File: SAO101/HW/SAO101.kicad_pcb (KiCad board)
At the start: 2 copper layers, 48 x 48 mm, 46 parts, among them J1 USB_B_Micro, J2 SAO_Conn, U1 AMS1117-3.3, U2 MCP23017_SS

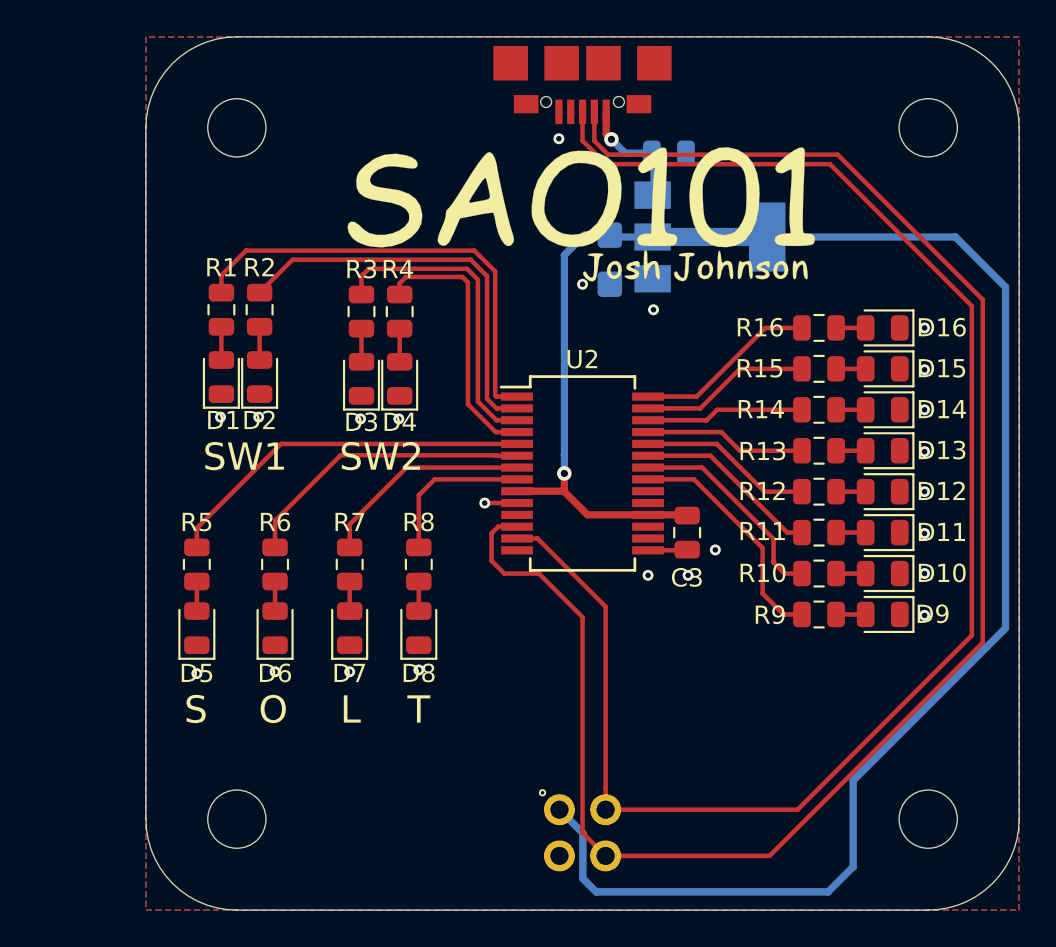
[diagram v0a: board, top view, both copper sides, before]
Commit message: add csides talk
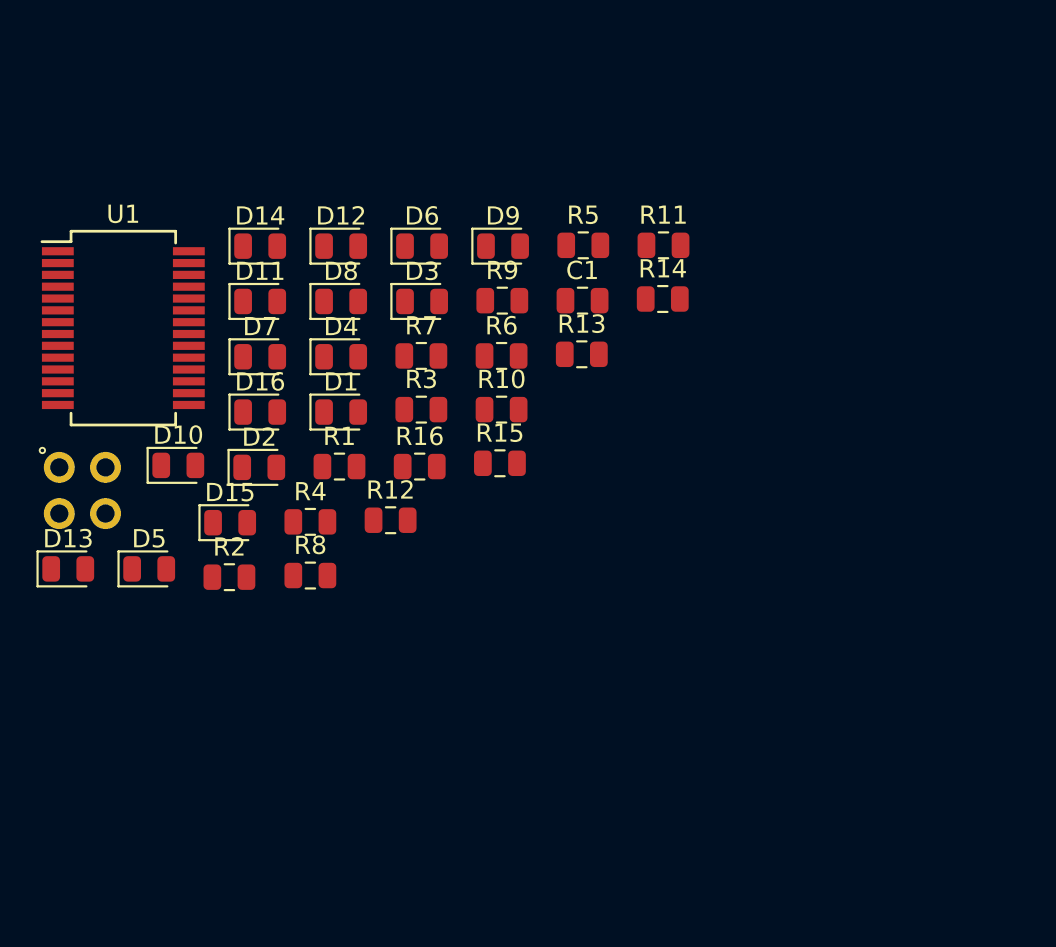
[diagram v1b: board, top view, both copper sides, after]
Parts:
- removed C2: 22u, Capacitor_Tantalum_SMD:CP_EIA-3216-18_Kemet-A
- removed C3: 100n, Capacitor_SMD:C_0805_2012Metric
- removed G***: LOGO, SAO101:josh_img
- removed G***: LOGO, SAO101:SAO101_img
- removed H1, H2, H3, H4: M3, MountingHole:MountingHole_3.2mm_M3_ISO14580
- removed J2: SAO_Conn, SAO101:SAO
- removed REF**: Josh Details, VNA_Footprints:JoshDetails
- removed U2: MCP23017_SS, Package_SO:SSOP-28_5.3x10.2mm_P0.65mm
- C1: value 10u -> 100n; moved to F.Cu
- J1: value USB_B_Micro -> SAO_Conn; footprint VNA_Footprints:MicroUSB_Aliexpress -> SAO101:SAO
- U1: value AMS1117-3.3 -> MCP23017_SS; footprint Package_TO_SOT_SMD:SOT-223-3_TabPin2 -> Package_SO:SSOP-28_5.3x10.2mm_P0.65mm; moved to F.Cu
- moved D13 45.2 mm to (98.7, 89.2), turned to 0 degrees
- moved D10 39.2 mm to (104.8, 83.6), turned to 0 degrees
- moved J1 37.1 mm to (99.5, 84.9), turned to 0 degrees
- moved D15 36.9 mm to (107.6, 86.7), turned to 0 degrees
- moved D11 36.5 mm to (109.3, 74.5), turned to 0 degrees
- moved D14 35.4 mm to (109.3, 71.5), turned to 0 degrees
- moved D16 34.5 mm to (109.3, 80.6), turned to 0 degrees
- moved D12 32.7 mm to (113.7, 71.5), turned to 0 degrees
- moved U1 32.6 mm to (101.8, 76.0)
- moved D9 29.1 mm to (122.6, 71.5), turned to 0 degrees
- moved R5 27.5 mm to (127.0, 71.5), turned to 0 degrees
- moved R9 24.5 mm to (122.6, 74.5), turned to 0 degrees
- moved R12 23.6 mm to (116.5, 86.6), turned to 0 degrees
- moved R16 23.2 mm to (118.0, 83.6), turned to 0 degrees
- moved D6 22.5 mm to (118.2, 71.5), turned to 0 degrees
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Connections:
- C1 pad 1: VBUS -> +3V3
- J1 pad 1: VBUS -> +3V3
- J1 pad 2: /SCL -> GND
- J1 pad 3: /SDA -> /SCL
- J1 pad 4: (no net) -> /SDA
- U1 pad 1: GND -> Net-(R1-Pad2)
- U1 pad 2: +3V3 -> Net-(R2-Pad2)
- U1 pad 3: VBUS -> Net-(R3-Pad2)
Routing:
- net +3V3: track 104.2 -> 0.00 mm, vias 1 -> 0
- net /SCL: track 94.0 -> 0.00 mm
- net /SDA: track 86.5 -> 0.00 mm
- net Net-(R1-Pad2): track 25.1 -> 0.00 mm
- net Net-(R2-Pad2): track 22.2 -> 0.00 mm
- net Net-(R5-Pad2): track 20.6 -> 0.00 mm
- net Net-(R3-Pad2): track 17.1 -> 0.00 mm
- net Net-(R6-Pad2): track 16.3 -> 0.00 mm
- net Net-(R4-Pad2): track 14.7 -> 0.00 mm
- net Net-(R9-Pad2): track 13.0 -> 0.00 mm
- net Net-(R7-Pad2): track 11.8 -> 0.00 mm
- net Net-(R10-Pad2): track 11.6 -> 0.00 mm
- net Net-(R11-Pad2): track 10.2 -> 0.00 mm
- net Net-(R16-Pad2): track 10.0 -> 0.00 mm
- net Net-(R12-Pad2): track 9.55 -> 0.00 mm
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- removed copper zone on B.Cu, net GND
- removed copper zone on F.Cu, net GND
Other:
- board outline removed
- rule pad_to_mask_clearance: 0.051 -> 0
- board text removed: "L"
- board text removed: "O"
- board text removed: "S"
- board text removed: "SW1"
- board text removed: "SW2"
- board text removed: "T"
